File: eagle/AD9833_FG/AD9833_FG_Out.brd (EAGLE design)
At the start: 27.6 x 38.1 mm, 12 parts, among them IC1 AD822N

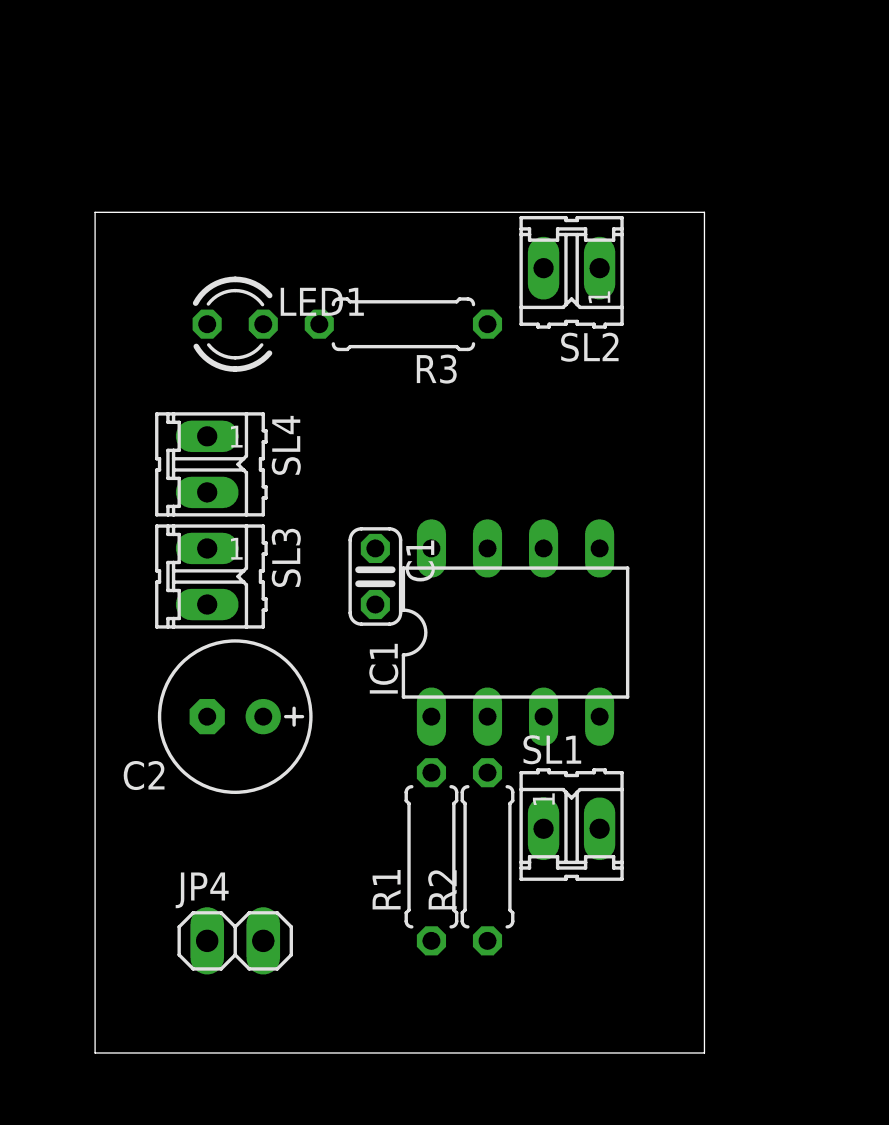
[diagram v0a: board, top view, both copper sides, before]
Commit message: Update eagle files
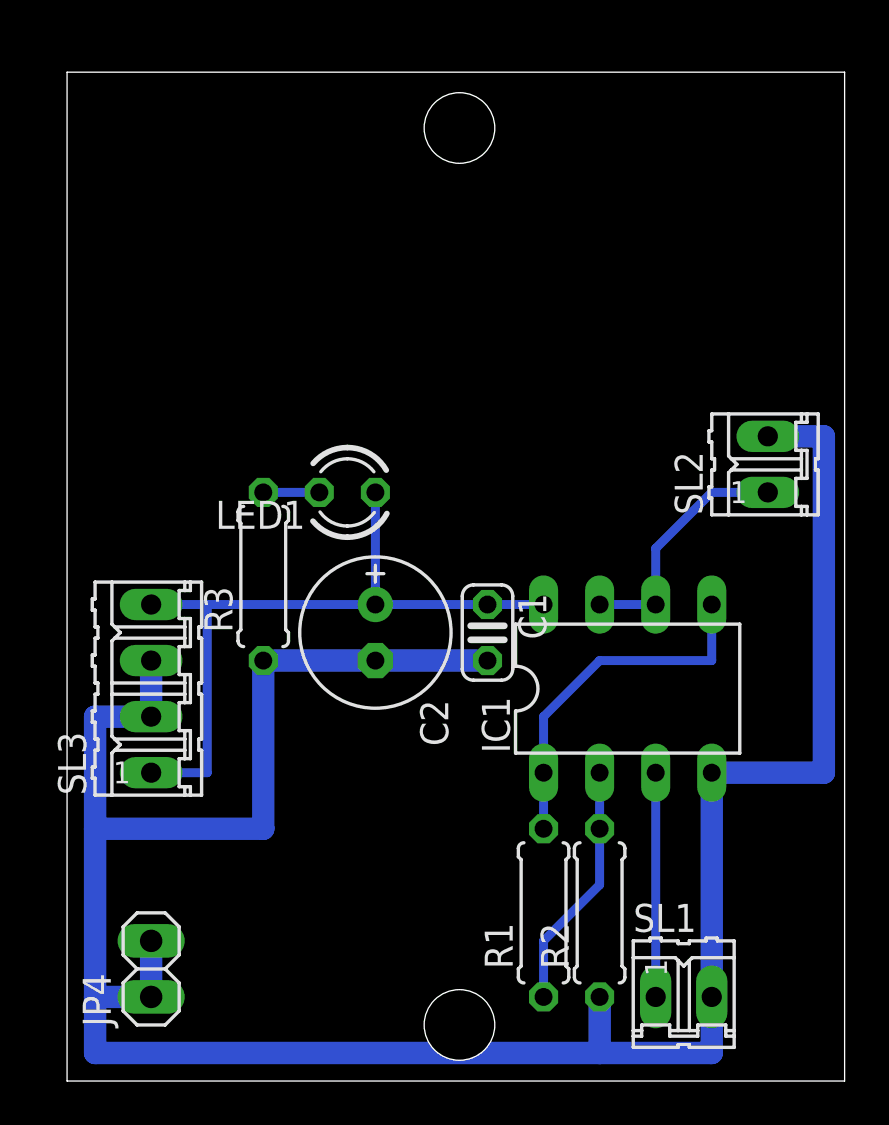
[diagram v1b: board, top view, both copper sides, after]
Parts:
- removed SL4: PWR, con-amp-quick:02P
- R3: value 4.7k -> 2.2k
- SL3: device con-amp-quick:02P -> con-amp-quick:04P
- moved R3 13.1 mm to (7.62, 21.6), turned to 90 degrees
- moved SL2 12.6 mm to (30.5, 26.7), turned to 90 degrees
- moved LED1 9.16 mm to (11.4, 25.4), turned to 180 degrees
- moved SL1 9.16 mm to (26.7, 2.54)
- moved C2 7.41 mm to (12.7, 19.1), turned to 270 degrees
- moved C1 5.68 mm to (17.8, 19.1)
- moved R1 5.68 mm to (20.3, 6.35)
- moved R2 5.68 mm to (22.9, 6.35)
- moved IC1 5.68 mm to (24.1, 16.5)
- moved SL3 5.68 mm to (2.54, 16.5), turned to 90 degrees
- moved JP4 4.02 mm to (2.54, 3.81), turned to 90 degrees
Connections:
- net AGND: now also SL2.2, SL3.2, SL3.3; no longer SL2.1, SL3.1, SL4.2
- net N$5: now also SL2.1; no longer SL2.2
- net V+: now also SL3.1, SL3.4; no longer SL3.2, SL4.1
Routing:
- net AGND: track 0.00 -> 118.1 mm
- net V+: track 0.00 -> 33.0 mm
- net N$4: track 0.00 -> 16.3 mm
- net N$5: track 0.00 -> 11.2 mm
- net N$1: track 0.00 -> 11.2 mm
- net N$2: track 0.00 -> 10.2 mm
- net N$8: track 0.00 -> 2.54 mm
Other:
- board size 27.6 x 38.1 mm -> 35.2 x 45.7 mm

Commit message: Impl. Amp Board
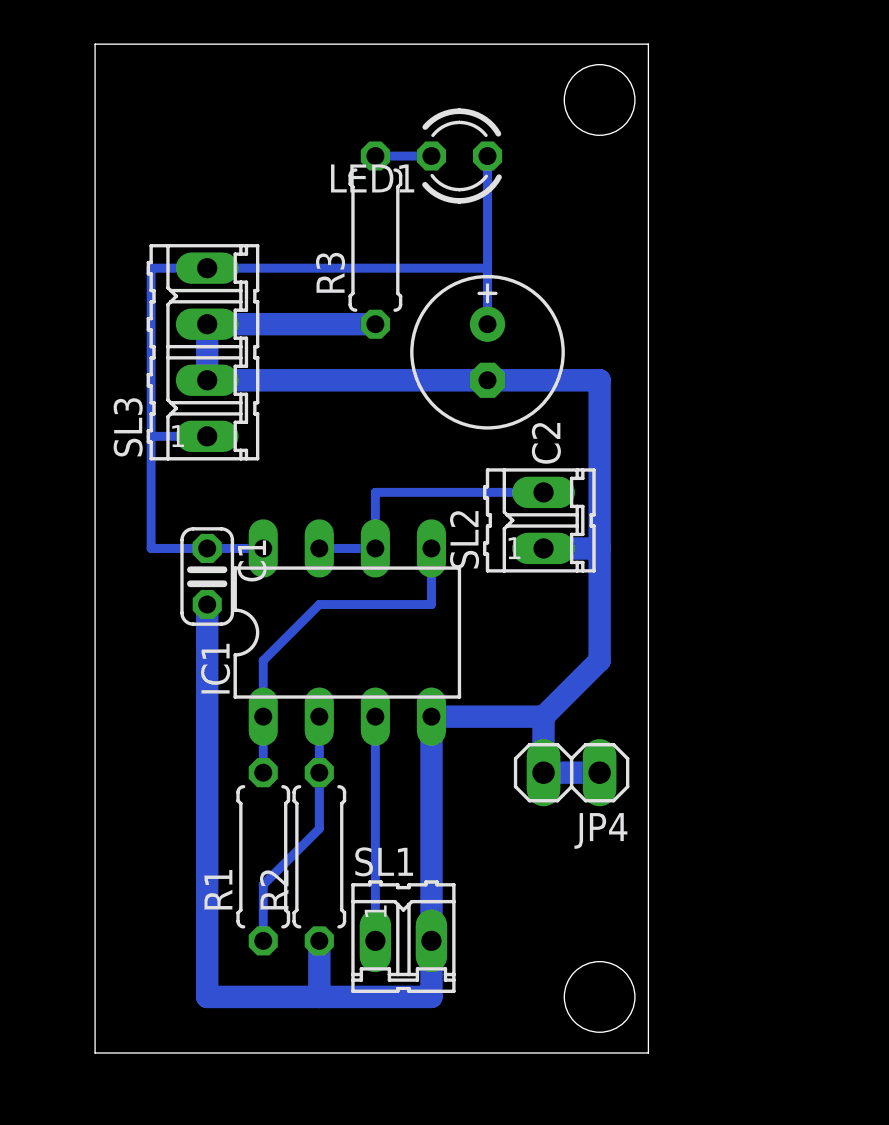
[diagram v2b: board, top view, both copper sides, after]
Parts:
- moved JP4 21.0 mm to (21.6, 12.7), turned to 180 degrees
- moved LED1 16.1 mm to (16.5, 40.6)
- moved R3 16.1 mm to (12.7, 36.8)
- moved SL3 15.5 mm to (5.08, 31.8)
- moved C2 13.7 mm to (17.8, 31.8)
- moved C1 13.0 mm to (5.08, 21.6)
- moved SL1 13.0 mm to (14.0, 5.08)
- moved IC1 13.0 mm to (11.4, 19.1)
- moved R1 13.0 mm to (7.62, 8.89)
- moved R2 13.0 mm to (10.2, 8.89)
- moved SL2 10.5 mm to (20.3, 24.1)
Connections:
- net AGND: now also SL2.1; no longer SL2.2
- net N$5: now also SL2.2; no longer SL2.1
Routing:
- net AGND: track 118.1 -> 100.1 mm
- net V+: track 33.0 -> 43.2 mm
- net N$5: track 11.2 -> 12.7 mm
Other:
- board size 35.2 x 45.7 mm -> 25.1 x 45.7 mm
